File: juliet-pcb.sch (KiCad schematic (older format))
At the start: 94 parts, among them SW0 KEYSW, SW1 KEYSW, SW10 KEYSW, SW11 KEYSW, SW12 KEYSW, SW13 KEYSW, SW14 KEYSW, SW15 KEYSW, SW16 KEYSW, SW17 KEYSW, SW18 KEYSW, SW19 KEYSW, SW2 KEYSW, SW20 KEYSW, SW21 KEYSW, SW22 KEYSW, SW23 KEYSW, SW24 KEYSW, SW25 KEYSW, SW26 KEYSW, SW27 KEYSW, SW28 KEYSW, SW29 KEYSW, SW3 KEYSW, SW30 KEYSW, SW31 KEYSW, SW32 KEYSW, SW33 KEYSW, SW34 KEYSW, SW35 KEYSW, SW36 KEYSW, SW37 KEYSW, SW38 KEYSW, SW39 KEYSW, SW4 KEYSW, SW40 KEYSW, SW41 KEYSW, SW42 KEYSW, SW43 KEYSW, SW44 KEYSW, SW45 KEYSW, SW46 KEYSW, SW47 KEYSW, SW5 KEYSW, SW6 KEYSW, SW7 KEYSW, SW8 KEYSW, SW9 KEYSW, U1 Pro_Micro

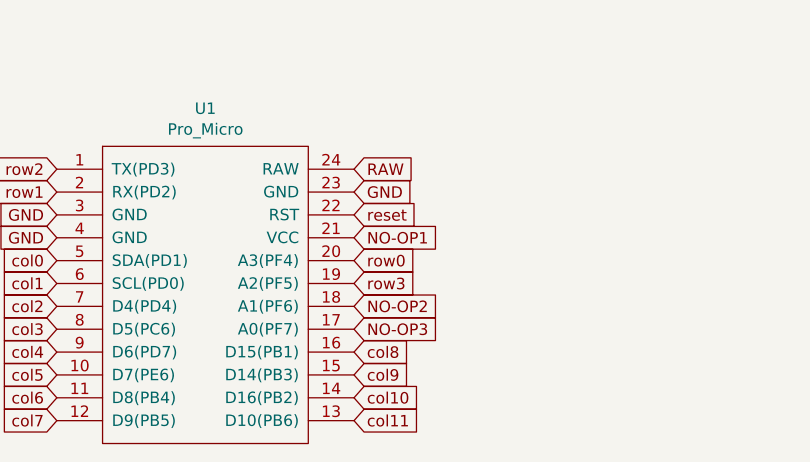
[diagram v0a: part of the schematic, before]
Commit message: Fixed a lot of issues.
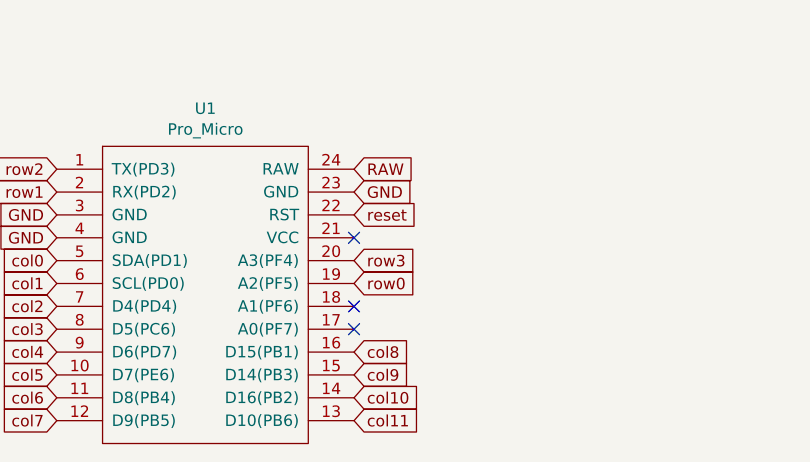
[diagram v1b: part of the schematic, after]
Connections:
- net row0: now also U1.19 (A2(PF5)); no longer U1.20 (A3(PF4))
- net row3: now also U1.20 (A3(PF4)); no longer U1.19 (A2(PF5))
- net NO-OP1: no longer names the net of U1.21 (VCC)
- net NO-OP2: no longer names the net of U1.18 (A1(PF6))
- net NO-OP3: no longer names the net of U1.17 (A0(PF7))
- no-connect marks 0 -> 3
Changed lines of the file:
@@
 Text GLabel 7200 4400 2    50   Input ~ 0
 GND
+Text GLabel 7200 4700 2    50   Input ~ 0
+row3
 Text GLabel 7200 4800 2    50   Input ~ 0
-row3
-Text GLabel 7200 4700 2    50   Input ~ 0
 row0
-Text GLabel 7200 4600 2    50   Input ~ 0
-NO-OP1
-Text GLabel 7200 4900 2    50   Input ~ 0
-NO-OP2
-Text GLabel 7200 5000 2    50   Input ~ 0
-NO-OP3
+NoConn ~ 7200 4600
+NoConn ~ 7200 4900
+NoConn ~ 7200 5000
 $EndSCHEMATC
